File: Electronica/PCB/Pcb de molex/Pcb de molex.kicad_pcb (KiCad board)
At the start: 2 copper layers, 73.1 x 52.6 mm, 11 parts, among them J1 Conn_01x05, J2 Conn_01x05, J3 Conn_01x05, U1 ULTRASONICO1, U2 ULTRASONICO2, U3 ULTRASONICO3, U4 ULTRASONICO4, U5 ULTRASONICO5

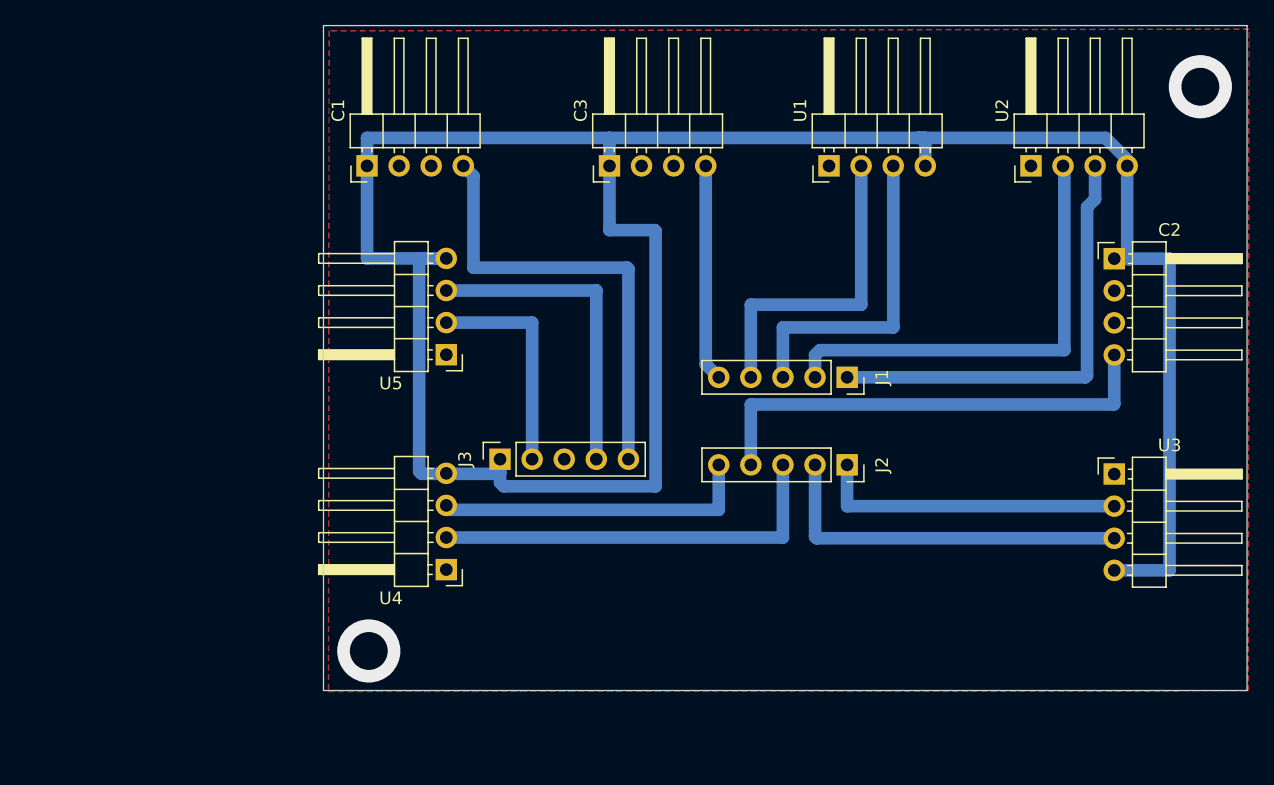
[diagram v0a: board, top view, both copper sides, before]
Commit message: ?
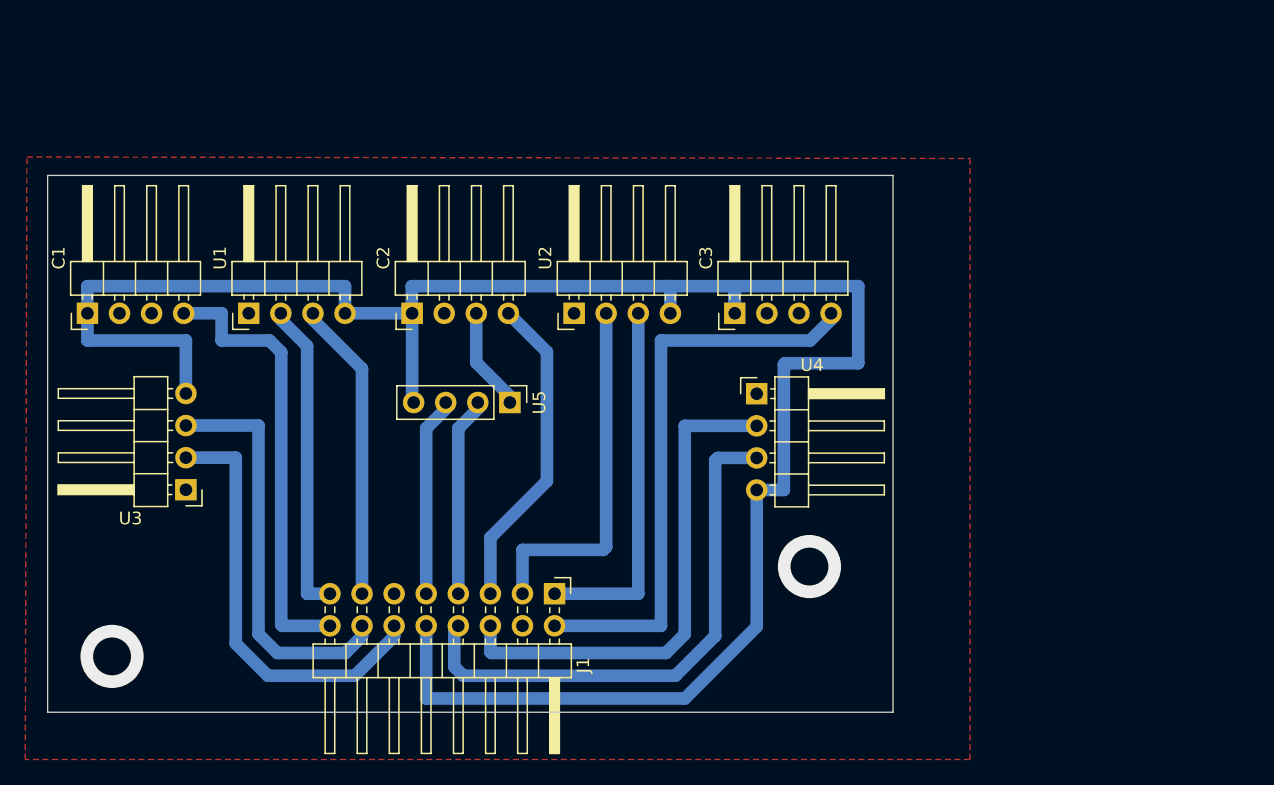
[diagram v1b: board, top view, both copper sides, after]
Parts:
- removed J2, J3: Conn_01x05, Connector_PinSocket_2.54mm:PinSocket_1x05_P2.54mm_Vertical
- J1: value Conn_01x05 -> Conn_02x08_Odd_Even; footprint Connector_PinSocket_2.54mm:PinSocket_1x05_P2.54mm_Vertical -> Connector_PinHeader_2.54mm:PinHeader_2x08_P2.54mm_Horizontal
- U5: footprint Connector_PinHeader_2.54mm:PinHeader_1x04_P2.54mm_Horizontal -> Connector_PinHeader_2.54mm:PinHeader_1x04_P2.54mm_Vertical
- moved U3 73.5 mm to (183.7, 66.9), turned to 180 degrees
- moved C2 55.7 mm to (201.6, 52.9), turned to 90 degrees
- moved U1 47.4 mm to (188.7, 52.9)
- moved U2 38.0 mm to (214.4, 52.9)
- moved J1 28.8 mm to (212.9, 75.1)
- moved U4 28.2 mm to (228.9, 59.3), turned to 0 degrees
- moved C1 25.0 mm to (175.9, 52.9)
- moved C3 15.3 mm to (227.2, 52.9)
- moved U5 6.30 mm to (209.4, 60.0), turned to -90 degrees
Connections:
- J1 pad 2: ECHO2 -> CNY3
- J1 pad 3: TRIG1 -> ECHO2
- J1 pad 4: ECHO1 -> unconnected-(J1-Pin_4-Pad4)
- J1 pad 5: CNY3 -> CNY2
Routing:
- net +5V: track 194.1 -> 164.2 mm
- net CNY3: track 17.2 -> 45.7 mm
- net TRIG4: track 25.3 -> 42.9 mm
- net CNY2: track 37.4 -> 25.3 mm
- net ECHO3: track 24.4 -> 34.4 mm
- net TRIG5: track 25.2 -> 15.8 mm
- net GND: track 0.00 -> 8.16 mm
- net ECHO4: track 32.4 -> 40.3 mm
- net ECHO2: track 36.3 -> 28.7 mm
- net TRIG2: track 35.9 -> 28.8 mm
- net TRIG3: track 29.4 -> 32.4 mm
- net ECHO5: track 17.6 -> 15.8 mm
- net TRIG1: track 25.5 -> 23.8 mm
- net ECHO1: track 25.5 -> 24.9 mm
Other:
- board size 73.1 x 52.6 mm -> 66.9 x 42.5 mm
